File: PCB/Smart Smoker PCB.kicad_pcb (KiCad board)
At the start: 4 copper layers, 90 x 45 mm, 76 parts, among them J1 105017-0001, J2 393570002, J3 393570002, J4 393570002, J5 393570002, J6 393570002, J7 Hopper, J8 Lid, Q1 Q_PMOS_GSD, Q2 25V 1.5A Trans, Q3 25V 1.5A Trans, Q4 Q_PMOS_GSD, Q5 2N7002T-7-F, Q6 2N7002T-7-F, U1 ESP32-WROOM-32UE_16MB, U2 DG409LEDY-T1-GE3, U3 MAX31855KASA, U4 AMS1117-3.3, U5 CP2102N-Axx-xQFN28, U6 LTC4412xS6

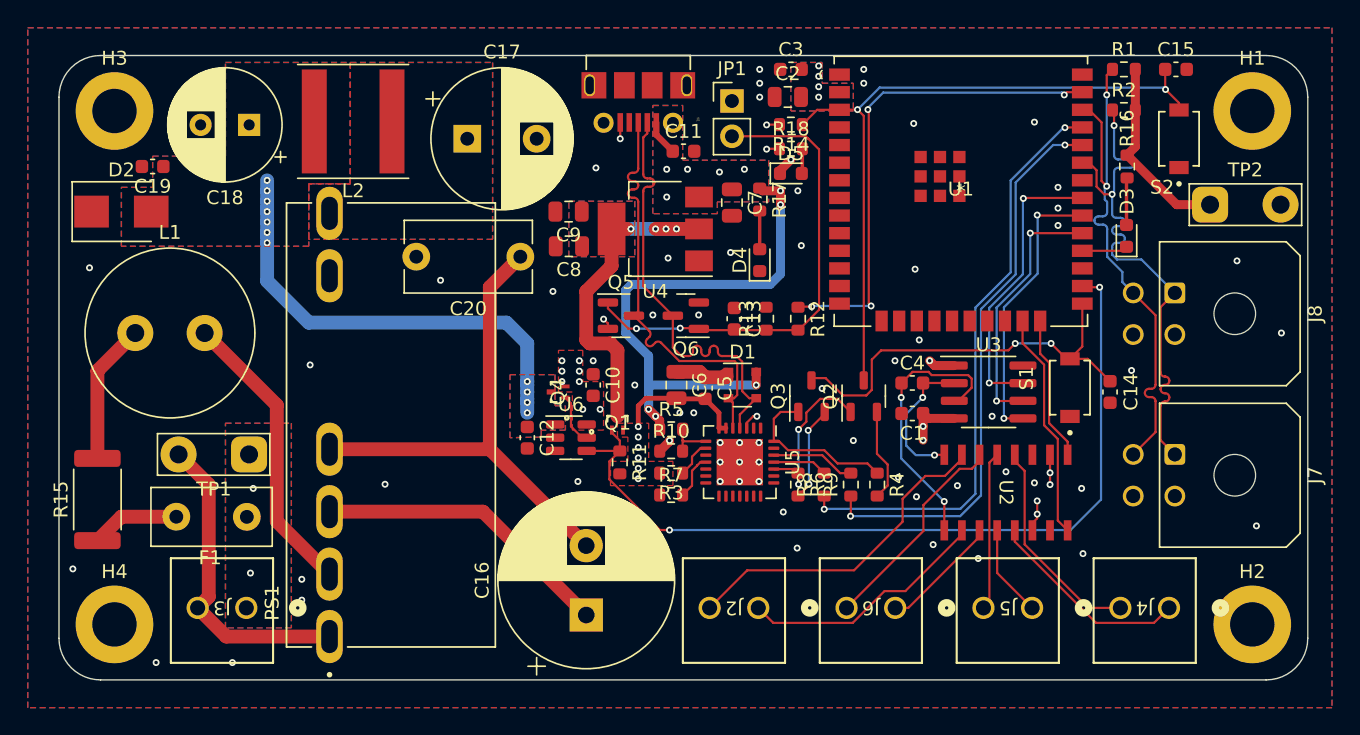
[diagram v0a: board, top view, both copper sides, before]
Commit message: Main pcb reviewed
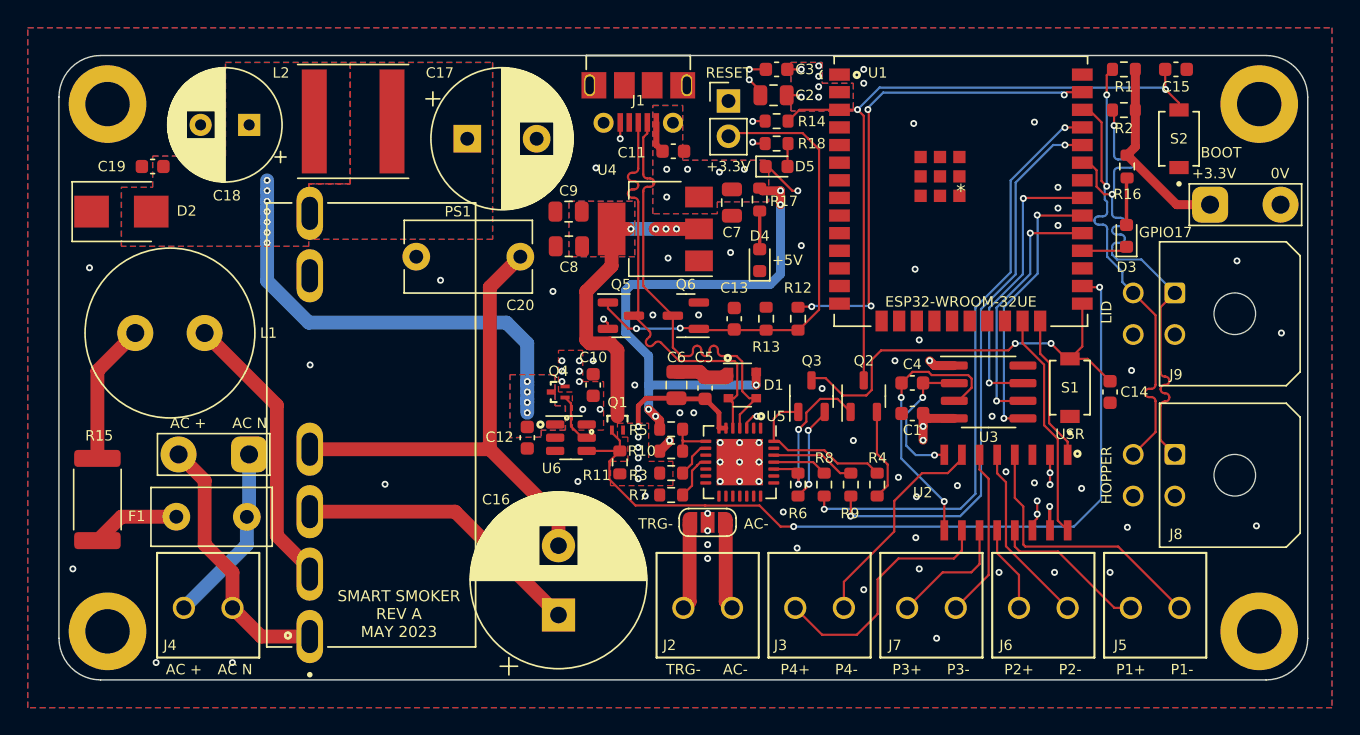
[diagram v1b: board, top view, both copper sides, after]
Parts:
- added J2: 393570002, Customs Smoker:CONN_393570002_MOL, F.Cu at (145.0, 139.8)
- added JP2: Jumper_3_Open, Jumper:SolderJumper-3_P1.3mm_Open_RoundedPad1.0x1.5mm, F.Cu at (146.8, 133.7)
- moved J4 4.50 mm to (109.0, 139.8), turned to 0 degrees
- moved J5 2.75 mm to (177.2, 139.8), turned to 0 degrees
- moved J3 2.66 mm to (153.1, 139.8), turned to 0 degrees
- moved C16 2.00 mm to (136.0, 140.3)
- moved PS1 1.42 mm to (118.1, 126.6)
- moved D5 1.14 mm to (151.7, 108.0)
- moved R18 1.10 mm to (151.7, 106.3)
- moved R14 1.06 mm to (151.7, 104.7)
- moved C2 1.04 mm to (151.5, 102.9)
- moved C3 1.03 mm to (151.7, 101.0)
- moved J6 0.95 mm to (169.2, 139.8), turned to 0 degrees
- moved J7 0.86 mm to (161.1, 139.8), turned to 0 degrees
- moved C11 0.73 mm to (144.3, 106.9)
- moved H1 0.71 mm to (186.5, 103.5)
- moved H2 0.71 mm to (186.5, 141.5)
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- renumbered J2 to J3, J3 to J4, J4 to J5, J5 to J6, J6 to J7, J7 to J8, J8 to J9
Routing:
- net /AC_L: track 0.00 -> 13.0 mm, vias 2 -> 0
- net /Probe4-: track 23.6 -> 15.6 mm
- net /AC_G: track 0.00 -> 6.35 mm
- net /TRG_GND: track 0.00 -> 6.35 mm
- net GND: track 11.6 -> 17.6 mm, vias 69 -> 76
- net /Probe1-: track 15.1 -> 19.9 mm
- net /AC_N: track 22.7 -> 19.1 mm
- net /Probe1+: track 14.8 -> 11.4 mm
- net /Probe3-: track 15.1 -> 12.3 mm
- net /Probe2-: track 10.8 -> 13.1 mm
- net +3.3V: track 33.5 -> 35.6 mm, vias 26 -> 28
- net /EN: track 50.4 -> 51.3 mm
- net /Probe3+: track 8.21 -> 8.96 mm
- net Net-(L1-Pad2): track 21.1 -> 20.4 mm
- net Net-(C16-Pad2): track 36.2 -> 36.8 mm
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- removed copper zone on B.Cu, net /AC_L
- removed copper zone on F.Cu, net /AC_L
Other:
- board text added: "+3.3V"
- board text added: "+5V"
- board text added: "0V"
- board text added: "90 x 45mm H M3x83x38mm"
- board text added: "AC +"
- board text added: "AC N"
- board text added: "AC-"
- board text added: "BOOT"
- board text added: "ESP32-WROOM-32UE"
- board text added: "GPIO17"
- board text added: "HOPPER"
- board text added: "LID"
- board text added: "P1+"
- board text added: "P1-"
- board text added: "P2+"
- board text added: "P2-"
- board text added: "P3+"
- board text added: "P3-"
- board text added: "P4+"
- board text added: "P4-"
- board text added: "RESET"
- board text added: "SMART SMOKER REV A MAY 2023"
- board text added: "Smart Smoker PCB REV A May 2023"
- board text added: "TRG-"
- board text added: "USR"
